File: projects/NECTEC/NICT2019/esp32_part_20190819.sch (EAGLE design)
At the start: 47 parts, among them Q1 BC847BS, U1 ESP-WROOM-32U (w/uFL), U2 IMAS980TH, U3 WG209_3E6, U4 RFM95W_SMT, X1 uFL, X2 uFL

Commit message: Almost finished the ESP32-CM3 design.
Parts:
- removed JP10: ANT1, microbuilder:HEADER-1X1ROUND
- removed JP11: Socket: 1U, pinhead:PINHD-2X18
- removed JP4: SDCARD_BREAKOUT, pinhead:PINHD-1X8
- removed JP5, JP6, JP7, JP8: JUMPER-SMT_3_NO_NO-SILK, ipas:JUMPER-SMT_3_NO_NO-SILK
- removed JP9: IM_SWD, pinhead:PINHD-1X4
- removed LED2: GREEN(0805), led:LEDCHIP-LED0805
- removed TP1, TP2, TP3, TP4: TPB1,27, ipas:TPB1,27
- removed U3: WG209_3E6, ipas:WG209
- removed X1: uFL, microbuilder:ANTENNA_U.FL
- added C18: 4.7uF, rcl:C-EUC1608
- added C8: 100nF, ipas:RCL_C-EUC1206
- added DD1: MAX487-S, rs232-rs485:MAX487-S
- added G1: CR2032V, battery:CR2032V
- added J2: MICRO-SD_CARD_SOCKETTINY, SparkFun-Connectors:MICRO-SD_CARD_SOCKETTINY
- added R13: 10k, ipas:RCL_R-USM0805
- added R14, R15, R16, R17: 100K, rcl:R-EU_R0603
- added RTC1: DS3231M, SparkFun-Clocks:DS3231M
- added SJ4, SJ5: (no value), ipas:SOLDERJUMPERREFLOW
- added SODIMM: RPI_COMPUTE, e14_Rpi_Compute_RevC:RPI_COMPUTE
- added TP_RFM_IO0, TP_RFM_IO1, TP_RFM_IO2, TP_RTC_32K, TP_RTC_INT: TPB1,27, ipas:TPB1,27
- C4: value 4.7uF -> 100nF; device ipas:RCL_CPOL-US150CLZ-1014 -> ipas:RCL_C-EUC1206
- R10, R12: value 100k -> 10k
- R5: value 100 -> 10k
- R7: value 100 -> 100k
- R9: value 470 -> 100k
- U2: value IMAS980TH -> BME280; device IMAS923TH:IMAS980TH -> SparkFun-Sensors:BME280
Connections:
- net ESP_GPIO2 renamed N$2
- net TX0_PRG renamed ESP_TX0
- removed net +5V: JP11.23, JP11.5
- removed net ADC1_0: TP1.TP, U1.SENSOR_VP
- removed net ADC1_3: TP2.TP, U1.SENSOR_VN
- removed net DAC1: TP3.TP, U1.IO25
- removed net IM_INT: R11.1, U1.IO35, U2.P11
- removed net IM_RST: JP9.3, R5.2, U2.!RESET
- removed net IM_RXD: U1.IO4, U2.RXD
- removed net IM_SWCLK: JP9.1, U2.P1/JTCK/SWCLK
- removed net IM_SWDAT: JP9.2, U2.P2/JTMS/SWDAT
- removed net IM_TXD: R12.1, U1.IO34, U2.TXD
- removed net N$1 (its old number): R9.2, U3.LED
- removed net N$2 (its old number): SJ3.1, U3.WPS
- removed net N$3: LED2.C, R9.1
- removed net NC14: JP11.14
- removed net NC16: JP11.16
- removed net PRTCTL1: JP11.21
- removed net RX0_PRG: JP3.1, U1.RXD0
- removed net RXD_TTL0: JP11.20, U1.IO17
- removed net SCL0_MID/RTC/CAM: JP11.7, U1.IO22
- removed net SCL_IO_EXP: JP11.24
- removed net SDA0_MID/RTC/CAM: JP11.9, U1.IO21
- removed net SDA_IO_EXP: JP11.26
- removed net SD_CLK: JP4.5, JP7.2
- removed net SD_CMD: JP4.3, JP6.2
- removed net SD_DAT0: JP4.7, JP8.2
- removed net SD_DAT1: JP4.8, SJ2.1
- removed net SD_DAT2: JP4.1, SJ1.1
- removed net SD_DAT3/CD: JP4.2, JP5.2
- removed net SPI1_CE0_1U: JP11.10
- removed net SPI1_CE1_1U: JP11.12, JP5.3
- removed net SPI1_MISO_1U: JP11.4, JP8.3
- removed net SPI1_MOSI_1U: JP11.6, JP6.3
- removed net SPI1_SCLK_1U: JP11.8, JP7.3
- removed net TXD_TTL0: JP11.18, R10.2, U1.IO16
- removed net USB_1N: JP11.17
- removed net USB_1P: JP11.19
- removed net USB_WN: JP11.13, U3.D-
- removed net USB_WP: JP11.15, U3.D+
- removed net WIFI_ON: JP11.11, SJ3.2
- new net 485_A: DD1G$1.A
- new net 485_B: DD1G$1.B
- new net AVCC: C5.1, U2.VDD
- new net CM_BCLK: SODIMM.63/GPIO18
- new net CM_DIN: SODIMM.71/GPIO21
- new net CM_DOUT: SODIMM.69/GPIO20
- new net CM_LRCIN: SODIMM.65/GPIO19
- new net CM_RX0_TERM: SODIMM.53/GPIO15
- new net CM_RX1: SODIMM.48/GPIO33
- new net CM_SCL0: SODIMM.5/GPIO1
- new net CM_SCL1: SODIMM.11/GPIO3
- new net CM_SDA0: SODIMM.3/GPIO0
- new net CM_SDA1: SODIMM.9/GPIO2
- new net CM_TX0_TERM: SODIMM.51/GPIO14
- new net CM_TX1: SODIMM.46/GPIO32
- new net CM_VDAC: SODIMM.189/VDAC, SODIMM.190/VDAC
- new net ESP_32K_XN: R12.1, RTC1.32KHZ, TP_RTC_32K.TP, U1.IO33
- new net ESP_32K_XP: C8.2, U1.IO32
- new net ESP_DIR_485: DD1G$1.DE, DD1G$1.RE/, U1.IO25
- new net ESP_RX0: JP3.1, R7.1, U1.RXD0
- new net ESP_RX1_AT: R9.1, SJ2.1, U1.IO16
- new net ESP_RX2_485: DD1G$1.RO, R11.1, U1.IO34
- new net ESP_TX1_AT: SJ1.1, U1.IO17
- new net ESP_TX2_485: DD1G$1.DI, U1.IO4
- new net GPIO5: SODIMM.17/GPIO5
- new net GPIO6: SODIMM.21/GPIO6
- new net HDMI_CEC: SODIMM.171/HDMI_CEC
- new net HDMI_CK_N: SODIMM.111/HDMI_CK_N*
- new net HDMI_CK_P: SODIMM.113/HDMI_CK_P*
- new net HDMI_D0_N: SODIMM.117/HDMI_D0_N*
- new net HDMI_D0_P: SODIMM.119/HDMI_D0_P*
- new net HDMI_D1_N: SODIMM.123/HDMI_D1_N*
- new net HDMI_D1_P: SODIMM.125/HDMI_D1_P*
- new net HDMI_D2_N: SODIMM.129/HDMI_D2_N*
- new net HDMI_D2_P: SODIMM.131/HDMI_D2_P*
- new net HDMI_HPD_N_1V8: SODIMM.88/GPIO46_1V8
- new net HDMI_SCL: SODIMM.175/HDMI_SCL
- new net HDMI_SDA: SODIMM.173/HDMI_SDA
- new net N$10: R14.2, SODIMM.30/GPIO29
- new net N$11: R17.2, SODIMM.82/GPIO44
- new net N$8: R16.2, SODIMM.84/GPIO45
- new net RPI_RX: SJ1.2
- new net RPI_SCL: SJ3.2
- new net RPI_SDA: SJ4.2
- new net RPI_TX: SJ2.2
- new net RTC_INT: R13.1, RTC1.SQW, TP_RTC_INT.TP, U1.IO35
- new net SCL0: R10.1, RTC1.SCL, SJ3.1, U1.IO22, U2.SCK/SCL
- new net SDA0: R5.1, RTC1.SDA, SJ4.1, U1.IO21, U2.SDI/SDA
- new net SDX_CLK: SODIMM.10/NC
- new net SDX_CMD: SODIMM.12/NC
- new net SDX_D0: SODIMM.16/NC
- new net SDX_D1: SODIMM.18/NC
- new net SDX_D2: SODIMM.22/NC
- new net SDX_D3: SODIMM.24/NC
- new net TV_DAC: SODIMM.166/TVDAC
- new net USB_DM: SODIMM.167/USB_DM**
- new net USB_DP: SODIMM.165/USB_DP**
- new net VCC_1V8: SODIMM.183/1V8, SODIMM.184/1V8, SODIMM.185/1V8, SODIMM.186/1V8
- new net VCC_3V3: C18.1, SODIMM.191/3V3, SODIMM.192/3V3, SODIMM.193/3V3, SODIMM.194/3V3, SODIMM.39/GPIO0-27_VREF, SODIMM.4/NC, SODIMM.40/GPIO0-27_VREF, SODIMM.41/GPIO28-45_VREF, SODIMM.42/GPIO28-45_VREF, SODIMM.6/NC
- new net VCC_5V: SODIMM.197/VBAT, SODIMM.198/VBAT, SODIMM.199/VBAT, SODIMM.200/VBAT
- net +3V3: now also C4.1, DD1G$2.VCC, J2.VCC, R10.2, R13.2, R5.2, R7.2, R9.2, RTC1.VCC, U2.!CS, U2.VDDIO; no longer C4.+, C5.1, JP11.1, JP4.4, LED2.A, R10.1, U2.VDD, U3.VCC
- net ESP_EN: now also SJ5.1
- net ESP_SD_CLK: now also J2.SCK; no longer JP7.1
- net ESP_SD_CMD: now also J2.DI; no longer JP6.1
- net ESP_SD_DAT0: now also J2.DO; no longer JP8.1
- net ESP_SD_DAT1: now also J2.RSV; no longer SJ2.2
- net ESP_SD_DAT2: now also J2.NC; no longer SJ1.2
- net ESP_SD_DAT3: now also J2.CS; no longer JP5.1
- net GND: now also C18.2, C4.2, C8.1, DD1G$2.GND, G1.-, J2.GND, J2.SHIELD, R14.1, R15.1, R16.1, R17.1, RTC1.GND, SODIMM.1/GND, SODIMM.103/GND, SODIMM.104/GND, SODIMM.109/GND, SODIMM.110/GND, SODIMM.115/GND, SODIMM.116/GND, SODIMM.121/GND, SODIMM.122/GND, SODIMM.127/GND, SODIMM.13/GND, SODIMM.133/GND, SODIMM.134/GND, SODIMM.139/GND, SODIMM.14/NC, SODIMM.140/GND, SODIMM.145/GND, SODIMM.146/GND, SODIMM.151/GND, SODIMM.152/GND, SODIMM.157/GND, SODIMM.163/GND, SODIMM.164/GND, SODIMM.168/USB_OTGID, SODIMM.169/GND, SODIMM.170/GND, SODIMM.181/GND, SODIMM.182/GND, SODIMM.187/GND, SODIMM.188/GND, SODIMM.19/GND, SODIMM.195/GND, SODIMM.196/GND, SODIMM.20/NC, SODIMM.25/GND, SODIMM.26/GND, SODIMM.31/GND, SODIMM.32/GND, SODIMM.37/GND, SODIMM.38/GND, SODIMM.43/GND, SODIMM.44/GND, SODIMM.49/GND, SODIMM.50/GND, SODIMM.55/GND, SODIMM.56/GND, SODIMM.61/GND, SODIMM.62/GND, SODIMM.67/GND, SODIMM.68/GND, SODIMM.7/GND, SODIMM.73/GND, SODIMM.74/GND, SODIMM.79/GND, SODIMM.8/NC, SODIMM.80/GND, SODIMM.85/GND, SODIMM.86/GND, SODIMM.91/GND, SODIMM.92/GND, SODIMM.97/GND, SODIMM.98/GND, U2.GND, U2.SDO/ADR; no longer C4.-, JP11.2, JP11.22, JP11.28, JP11.3, JP11.30, JP11.32, JP4.6, JP9.4, U2.GND@0, U2.GND@1, U2.GND@2, U2.GND@3, U2.GND@4, U2.GND@5, U2.GND@6, U2.GND@7, U3.GND, X1.GND@0, X1.GND@1
- net N$4: now also G1.+, RTC1.VBAT; no longer TP4.TP, U2.P16/BOOT0
- net N$5: now also RTC1.RST, SJ5.2; no longer R7.2, U2.P15/WKUP1/ADC_IN0
- net N$9: now also R15.2, SODIMM.28/GPIO28; no longer JP10.1, U2.RF, X1.SIGNAL
- net RFM_CS: no longer R7.1
- net RFM_IO0: now also TP_RFM_IO0.TP
- net RFM_IO1: now also TP_RFM_IO1.TP, U1.SENSOR_VN; no longer U1.IO33
- net RFM_IO2: now also TP_RFM_IO2.TP, U1.SENSOR_VP; no longer U1.IO32
- net RFM_RST: no longer R5.1
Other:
- note added: "Description: JRTU"
- note added: "ESP32 features three UARTs: UART0 -- for programming TX: IO1 RX: IO3 UART1 -- for AT-command service TX: IO17 RX: IO16 UART2 TX: IO4 RX: IO34 (34..39 is input only)"
- note added: "https://www.raspberrypi.org/documentation/hardware/computemodule/cmio-camera.md"
- note removed: "- WIFI_ON --> on/off the wifi module. - USB_WP, USB_WN --> D+,D- of the wifi module. - PRTCTL1 --> USB power on/off. - USB_1P, USB_1N --> D+,D- of the external USB."
- note removed: "Description: The communication module is meant to be a data gateway for uRTU and LRTU. Its functions are accomprised of: 1) 802.11 Wifi, 2) LoRaWAN, and 3) Micro SDCard interfacings."
- note removed: "ESP32 features three UARTs: UART0 -- for programming RX: IO3 TX: IO1 UART1 -- for AT-command service RX: IO16 TX: IO17 UART2 -- for eMOD RX: IO34 TX: IO4"

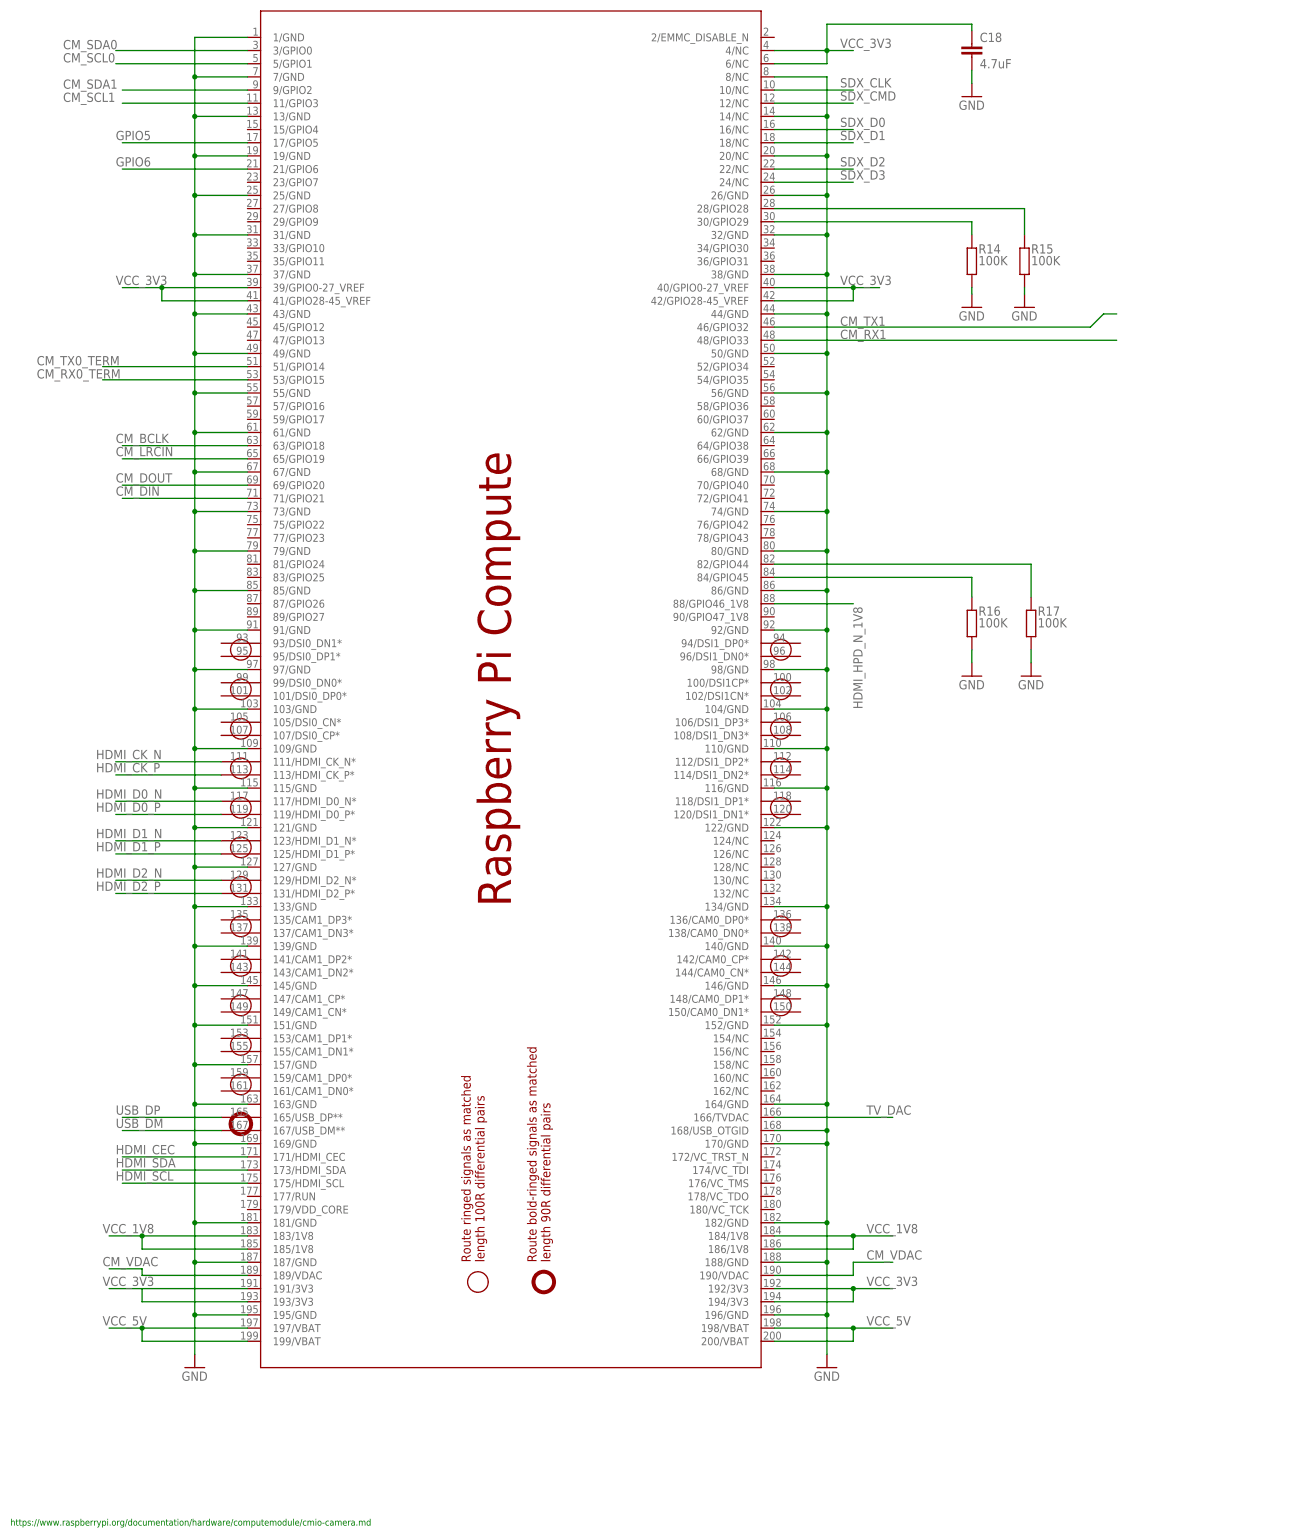
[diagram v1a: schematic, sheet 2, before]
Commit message: Complete the CM3-ESP32 board roughly.
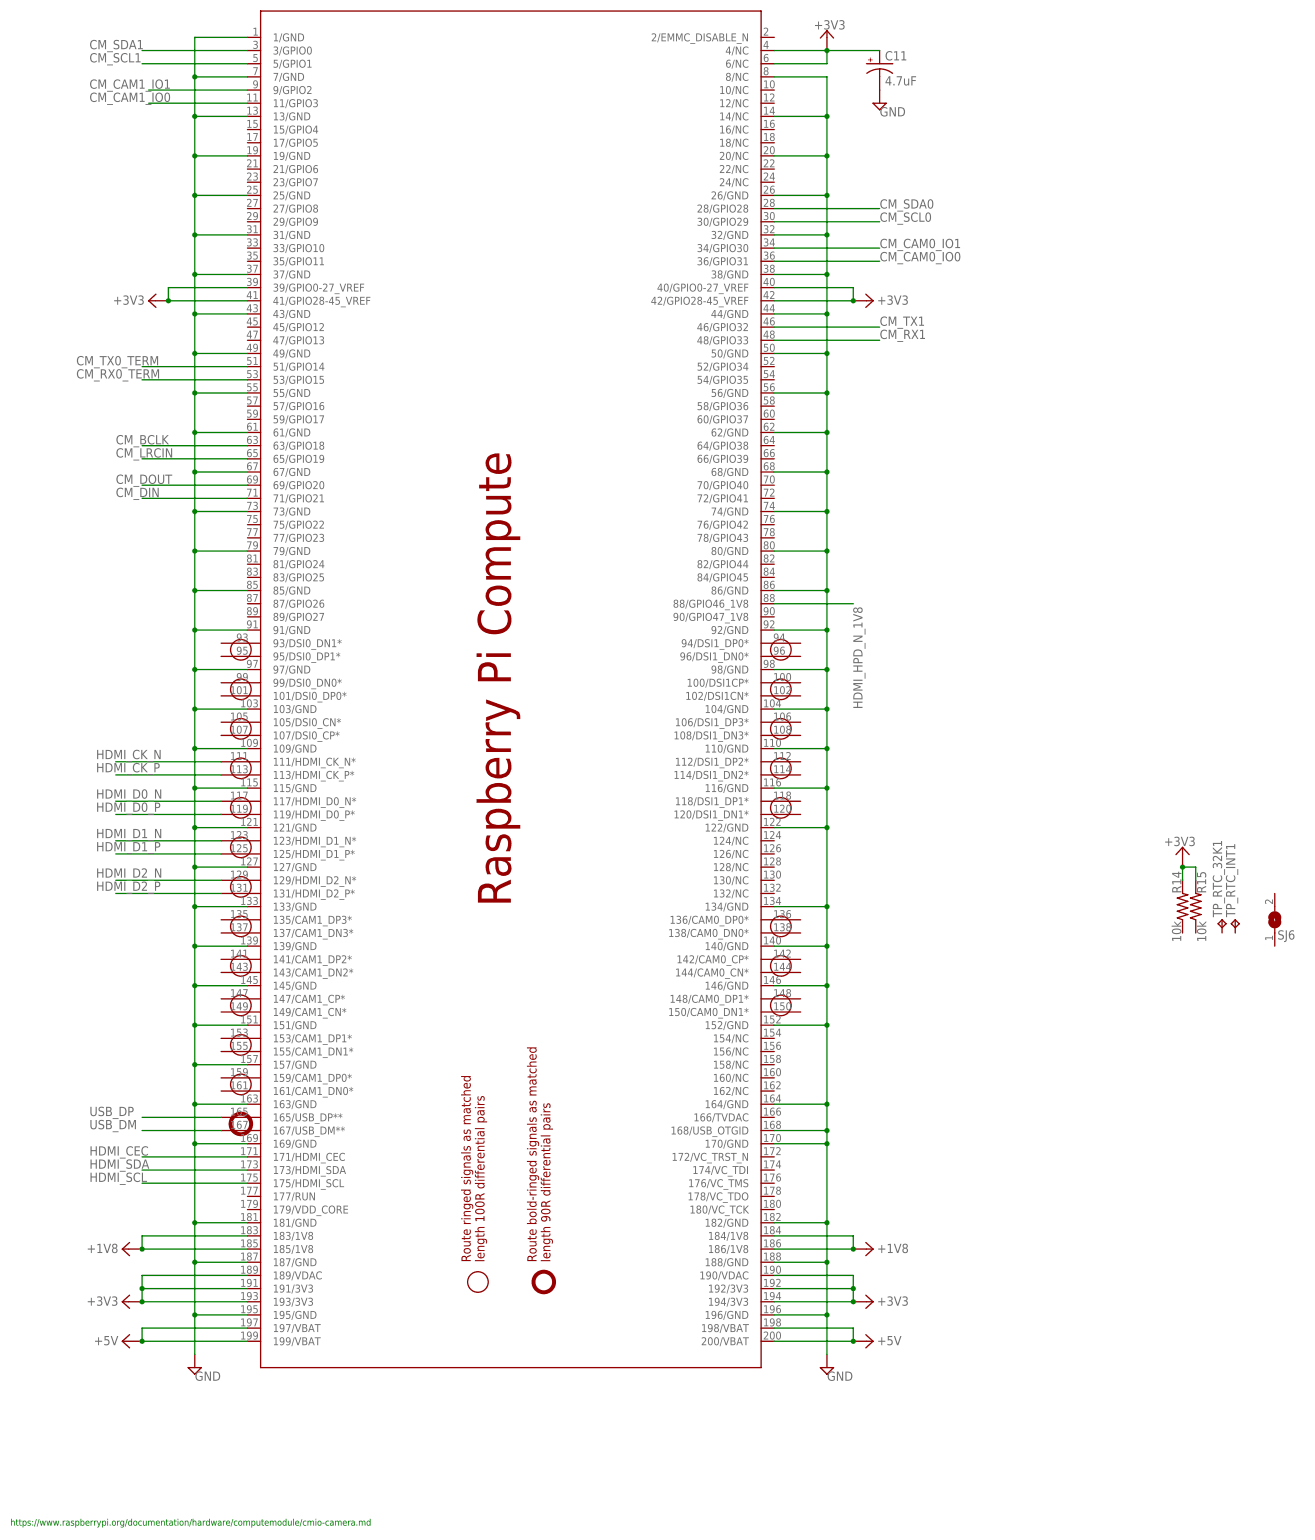
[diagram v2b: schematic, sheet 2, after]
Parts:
- removed C18: 4.7uF, rcl:C-EUC1608
- removed R16, R17: 100K, rcl:R-EU_R0603
- added C11: 4.7uF, ipas:RCL_CPOL-US150CLZ-1014
- added SJ6: (no value), ipas:SOLDERJUMPERREFLOW
- added TP_RTC_32K1, TP_RTC_INT1: TPB1,27, ipas:TPB1,27
- R14, R15: value 100K -> 10k; device rcl:R-EU_R0603 -> ipas:RCL_R-USM0805; CID 157 -> (none)
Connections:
- net VCC_5V renamed +5V
- removed net CM_VDAC: SODIMM.189/VDAC, SODIMM.190/VDAC
- removed net GPIO5: SODIMM.17/GPIO5
- removed net GPIO6: SODIMM.21/GPIO6
- removed net N$10: R14.2, SODIMM.30/GPIO29
- removed net N$11: R17.2, SODIMM.82/GPIO44
- removed net N$8: R16.2, SODIMM.84/GPIO45
- removed net N$9: R15.2, SODIMM.28/GPIO28
- removed net SDX_CLK: SODIMM.10/NC
- removed net SDX_CMD: SODIMM.12/NC
- removed net SDX_D0: SODIMM.16/NC
- removed net SDX_D1: SODIMM.18/NC
- removed net SDX_D2: SODIMM.22/NC
- removed net SDX_D3: SODIMM.24/NC
- removed net TV_DAC: SODIMM.166/TVDAC
- removed net VCC_1V8: SODIMM.183/1V8, SODIMM.184/1V8, SODIMM.185/1V8, SODIMM.186/1V8
- removed net VCC_3V3: C18.1, SODIMM.191/3V3, SODIMM.192/3V3, SODIMM.193/3V3, SODIMM.194/3V3, SODIMM.39/GPIO0-27_VREF, SODIMM.4/NC, SODIMM.40/GPIO0-27_VREF, SODIMM.41/GPIO28-45_VREF, SODIMM.42/GPIO28-45_VREF, SODIMM.6/NC
- new net CM_CAM0_IO0: SODIMM.36/GPIO31
- new net CM_CAM0_IO1: SODIMM.34/GPIO30
- new net CM_CAM1_IO0: SODIMM.11/GPIO3
- new net CM_CAM1_IO1: SODIMM.9/GPIO2
- net +3V3: now also C11.+, R14.2, R15.2, SODIMM.183/1V8, SODIMM.184/1V8, SODIMM.185/1V8, SODIMM.186/1V8, SODIMM.189/VDAC, SODIMM.190/VDAC, SODIMM.191/3V3, SODIMM.192/3V3, SODIMM.193/3V3, SODIMM.194/3V3, SODIMM.39/GPIO0-27_VREF, SODIMM.4/NC, SODIMM.40/GPIO0-27_VREF, SODIMM.41/GPIO28-45_VREF, SODIMM.42/GPIO28-45_VREF, SODIMM.6/NC
- net CM_SCL0: now also SODIMM.30/GPIO29; no longer SODIMM.5/GPIO1
- net CM_SCL1: now also SODIMM.5/GPIO1; no longer SODIMM.11/GPIO3
- net CM_SDA0: now also SODIMM.28/GPIO28; no longer SODIMM.3/GPIO0
- net CM_SDA1: now also SODIMM.3/GPIO0; no longer SODIMM.9/GPIO2
- net GND: now also C11.-; no longer C18.2, R14.1, R15.1, R16.1, R17.1
